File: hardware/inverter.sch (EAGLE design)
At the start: 51 parts, among them IC1 MEGA8-P, IC2 7805T, K1 ZF112, K2 ZF112, Q5 BC327, Q6 BC327

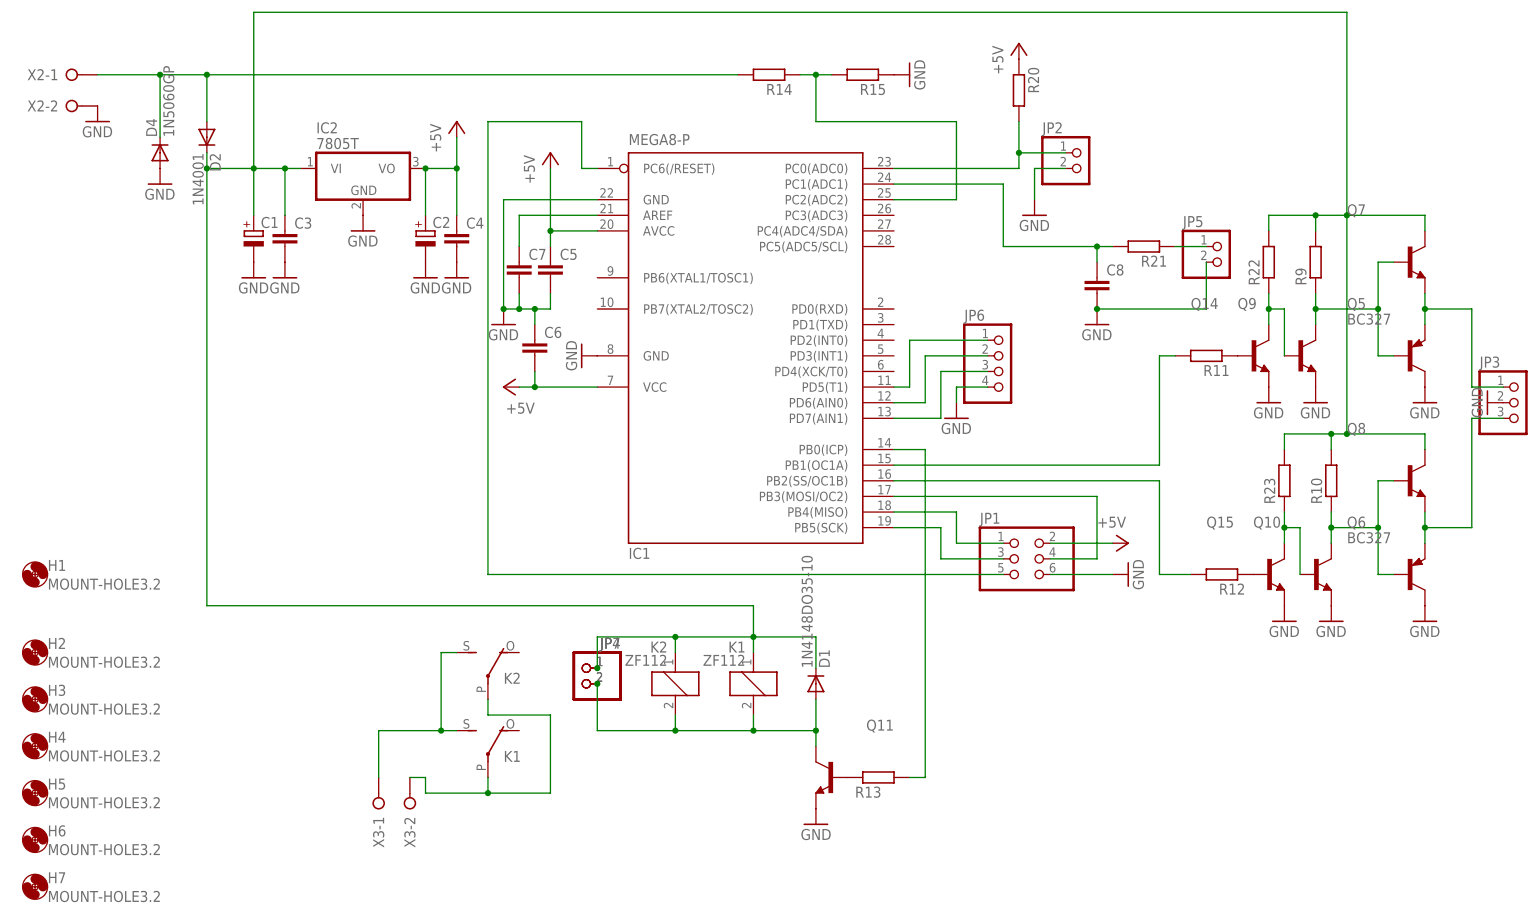
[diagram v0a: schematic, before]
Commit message: Added gitignore
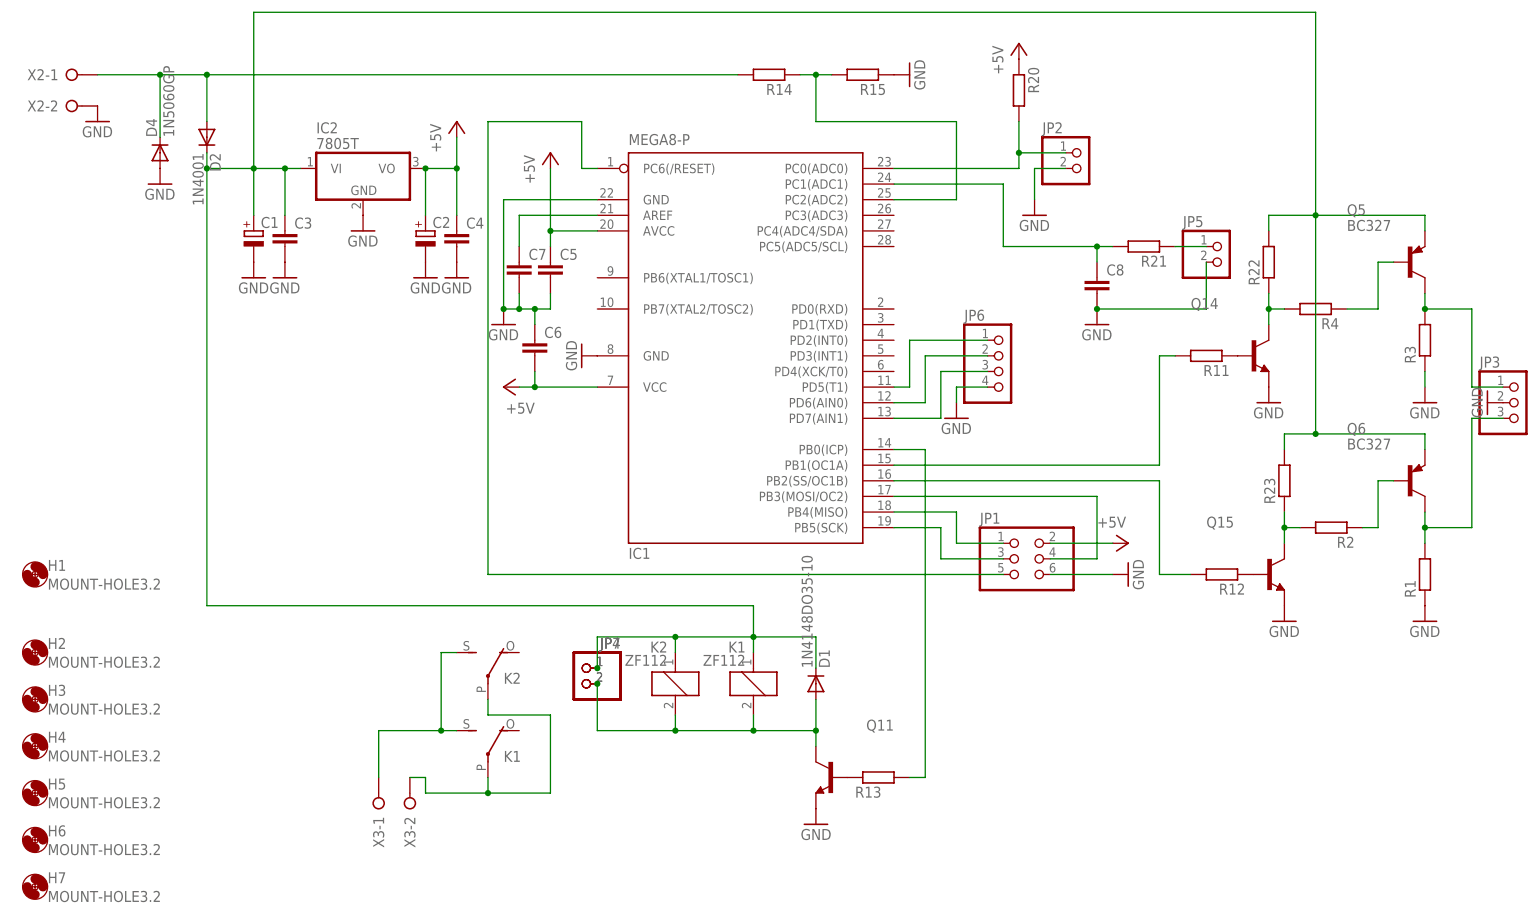
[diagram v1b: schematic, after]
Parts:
- removed Q10, Q9: (no value), transistor:BC547-NPN-TO92-CBE
- removed Q7: (no value), transistor:BC337-16-NPN-TO92-CBE
- removed Q8: (no value), transistor:BC237-NPN-TO92-CBE
- removed R10, R9: (no value), resistor:R-EU_0207/10
- added R1, R3: (no value), resistor:R-EU_0207/5V
- added R2, R4: (no value), resistor:R-EU_0207/2V
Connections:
- removed net N$15: Q10.C, Q6.B, Q8.B, R10.1
- removed net N$18: Q5.B, Q7.B, Q9.C, R9.1
- new net N$2: Q6.B, R2.1
- new net N$3: Q5.B, R4.1
- net GND: now also R1.1, R3.1; no longer Q10.E, Q5.C, Q6.C, Q9.E
- net N$13: now also Q6.C, R1.2; no longer Q6.E, Q8.E
- net N$19: now also R2.2; no longer Q10.B
- net N$26: now also Q5.E, Q6.E; no longer Q7.C, Q8.C, R10.2, R9.2
- net N$42: now also R4.2; no longer Q9.B
- net N$6: now also Q5.C, R3.2; no longer Q5.E, Q7.E
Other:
- moved on the sheet: Q5, Q6
